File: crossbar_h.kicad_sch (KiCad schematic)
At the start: 64 parts, among them U100 AD5160, U101 AD5160, U102 AD5160, U103 AD5160, U104 AD5160, U105 AD5160, U106 AD5160, U107 AD5160, U108 AD5160, U109 AD5160, U110 AD5160, U111 AD5160, U112 AD5160, U113 AD5160, U114 AD5160, U115 AD5160, U116 AD5160, U117 AD5160, U118 AD5160, U119 AD5160, U120 AD5160, U121 AD5160, U122 AD5160, U123 AD5160, U124 AD5160, U125 AD5160, U126 AD5160, U127 AD5160, U128 AD5160, U129 AD5160, U130 AD5160, U131 AD5160

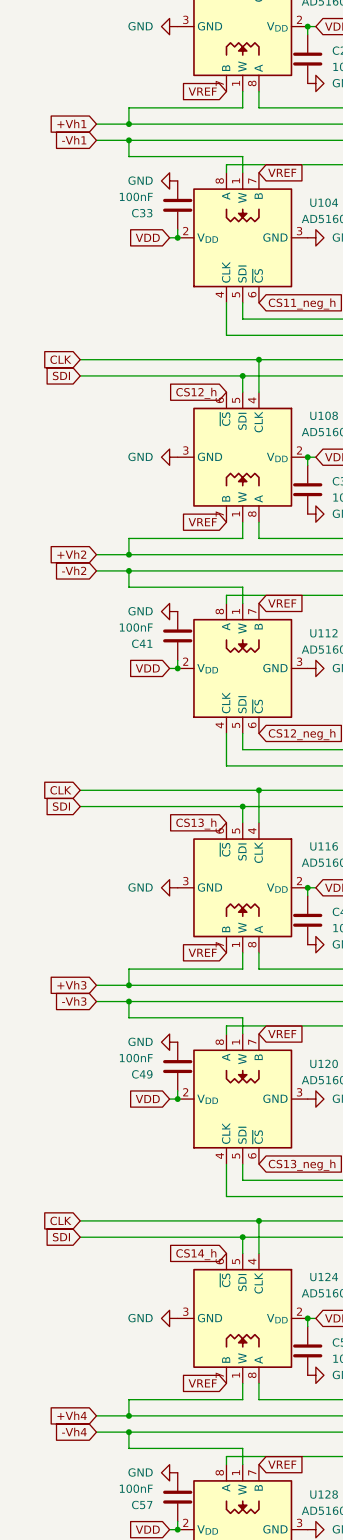
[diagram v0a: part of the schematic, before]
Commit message: Updated: PCB
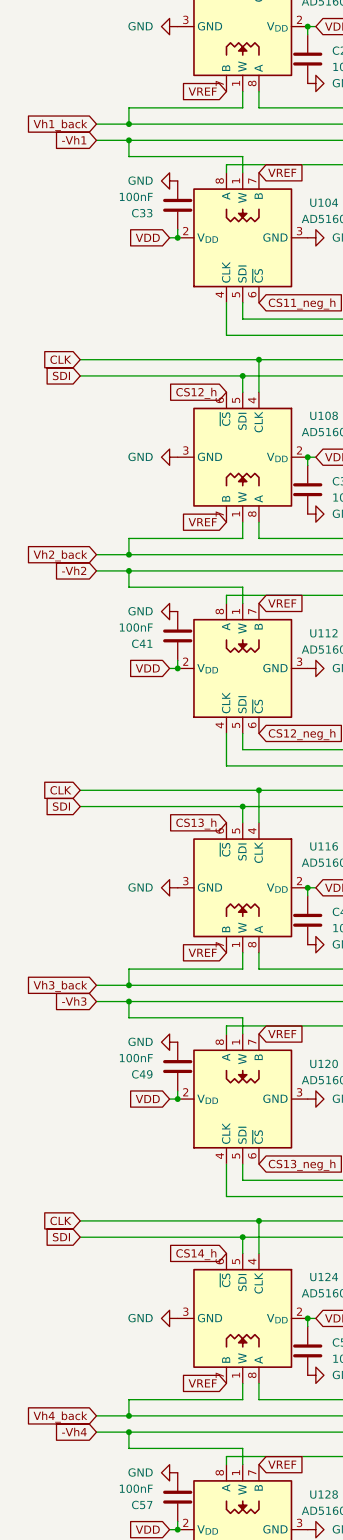
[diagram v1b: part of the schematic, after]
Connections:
- net +Vh1 renamed Vh1_back
- net +Vh2 renamed Vh2_back
- net +Vh3 renamed Vh3_back
- net +Vh4 renamed Vh4_back
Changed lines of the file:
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@@
 		)
 	)
-	(global_label "+Vh4"
+	(global_label "Vh4_back"
 		(shape input)
 		(at 73.66 298.45 180)
@@
 		)
 		(property "Intersheetrefs" "${INTERSHEET_REFS}"
-			(at 65.6553 298.45 0)
+			(at 61.8454 298.45 0)
 			(effects
 				(font
@@
 		)
 	)
-	(global_label "+Vh1"
+	(global_label "Vh1_back"
 		(shape input)
 		(at 73.66 96.52 180)
@@
 		)
 		(property "Intersheetrefs" "${INTERSHEET_REFS}"
-			(at 65.6553 96.52 0)
+			(at 61.8454 96.52 0)
 			(effects
 				(font
@@
 		)
 	)
-	(global_label "+Vh3"
+	(global_label "Vh3_back"
 		(shape input)
 		(at 73.66 231.14 180)
@@
 		)
 		(property "Intersheetrefs" "${INTERSHEET_REFS}"
-			(at 65.6553 231.14 0)
+			(at 61.8454 231.14 0)
 			(effects
 				(font
@@
 		)
 	)
-	(global_label "+Vh2"
+	(global_label "Vh2_back"
 		(shape input)
 		(at 73.66 163.83 180)
@@
 		)
 		(property "Intersheetrefs" "${INTERSHEET_REFS}"
-			(at 65.6553 163.83 0)
-			(effects
-				(font
+			(at 61.8454 163.83 0)
+			(effects
+				(font
